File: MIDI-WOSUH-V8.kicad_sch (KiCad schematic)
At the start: 17 parts, among them J1 Conn_01x02_Socket, J2 Conn_01x02_Socket, J3 Conn_01x02_Socket, J4 Conn_01x02_Socket, J5 Conn_01x02_Socket, J6 Conn_01x02_Socket, J7 Conn_01x02_Socket, J8 Conn_01x02_Socket, SW1 SW_Push, SW2 SW_Push, SW3 SW_Push, SW4 SW_Push

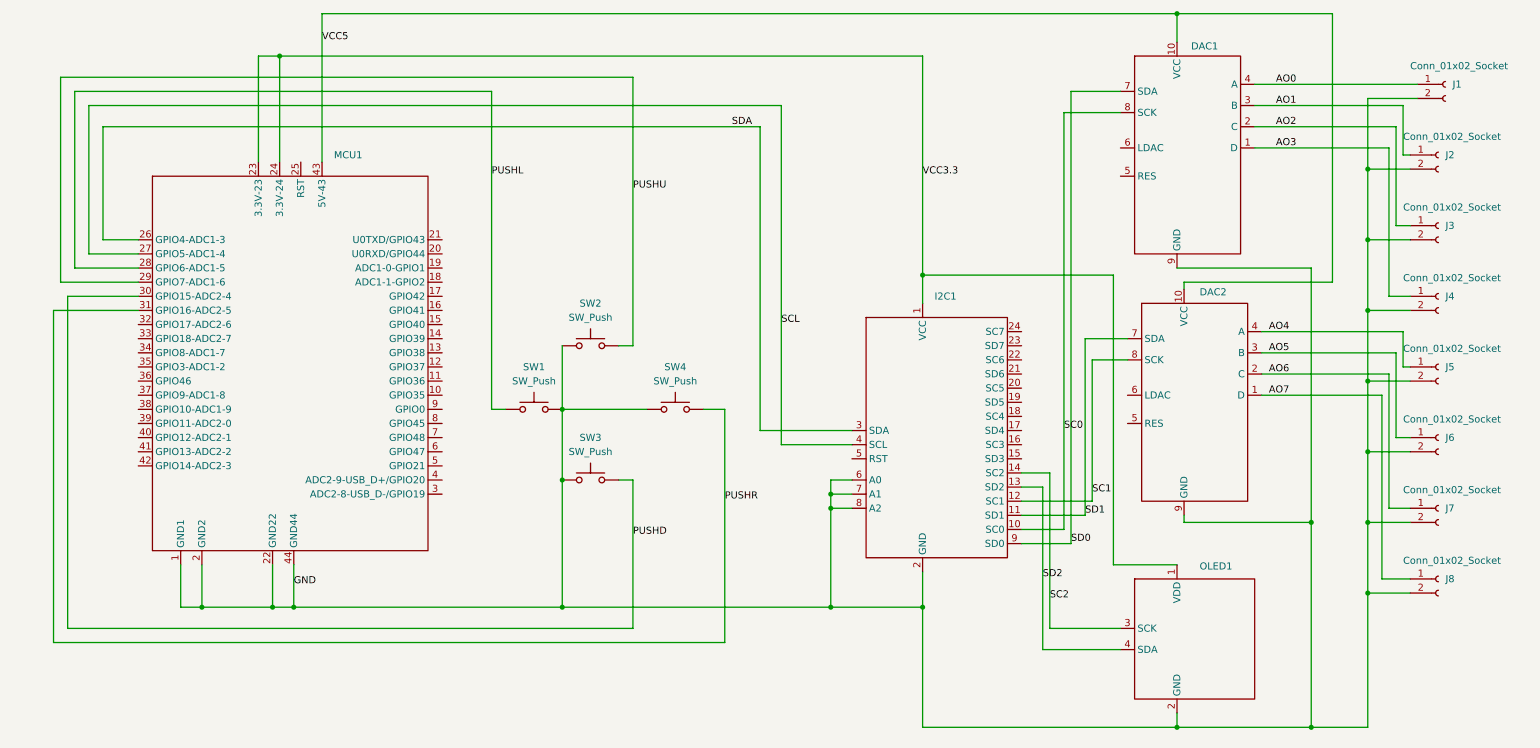
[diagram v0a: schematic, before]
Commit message: Add files via upload
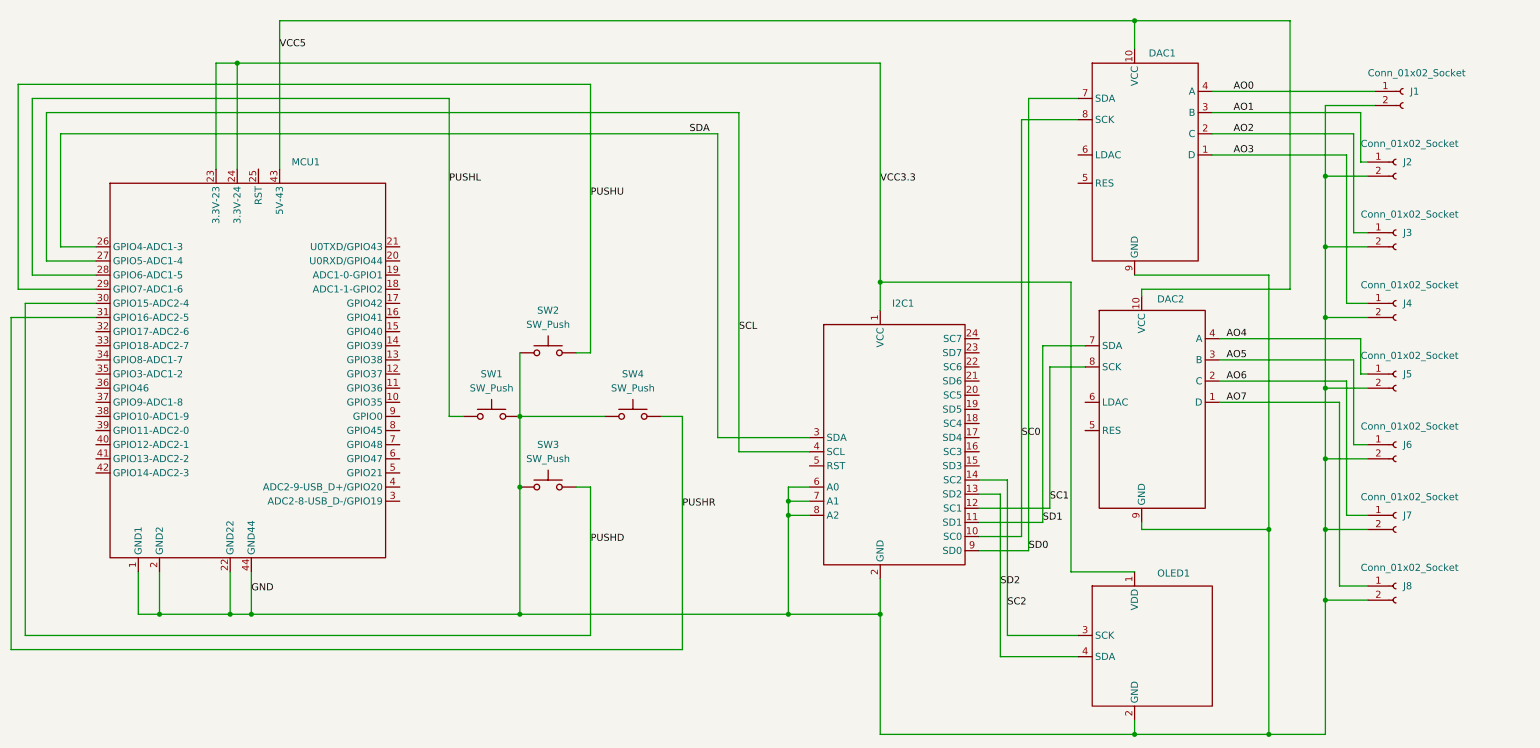
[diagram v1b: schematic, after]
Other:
- company: (none) -> Tutorius GbR
- title: (none) -> MIDIWOUSH V8 Schaltplan
- moved on the sheet: DAC1, DAC2, I2C1, J1, J2, J3, J4, J5, J6, J7, J8, MCU1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
